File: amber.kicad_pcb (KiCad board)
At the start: 2 copper layers, 118.9 x 112.3 mm, 50 parts, among them J1 SJ-43504-SMT-TR

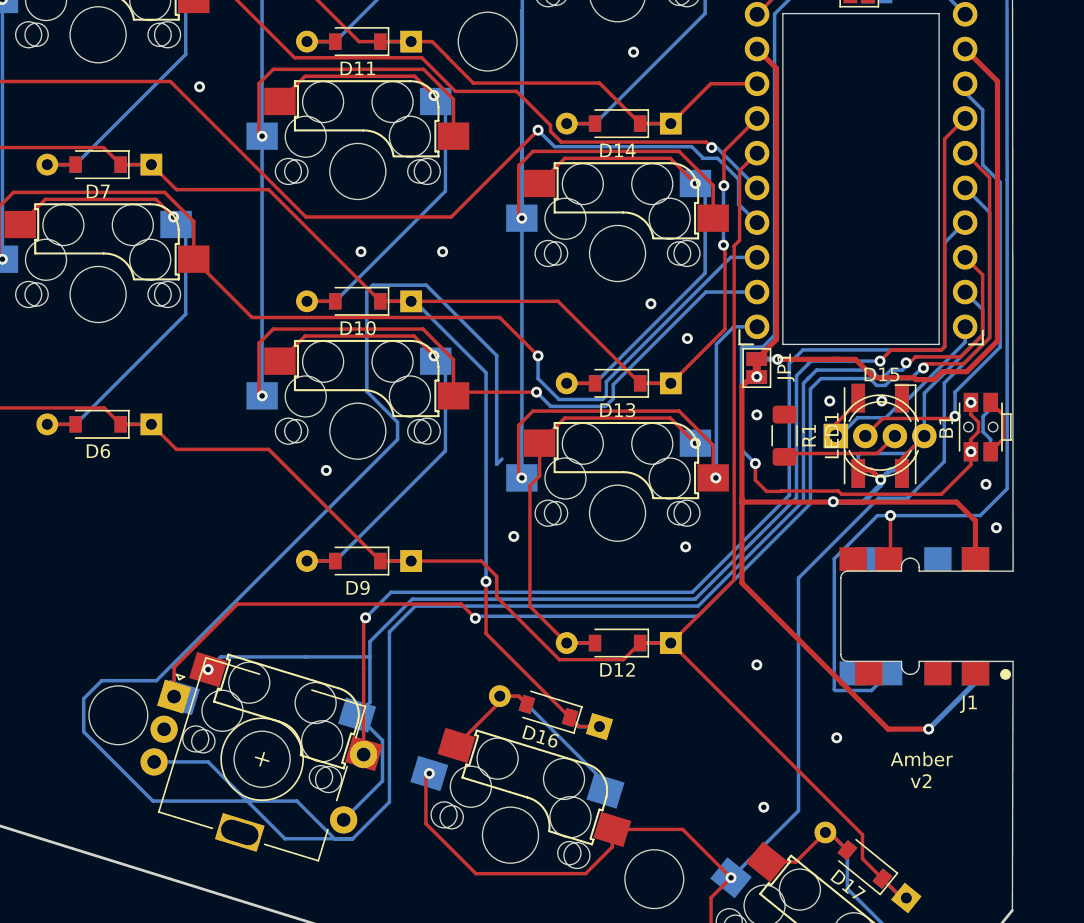
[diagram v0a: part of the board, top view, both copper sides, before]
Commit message: Cleanup tracks
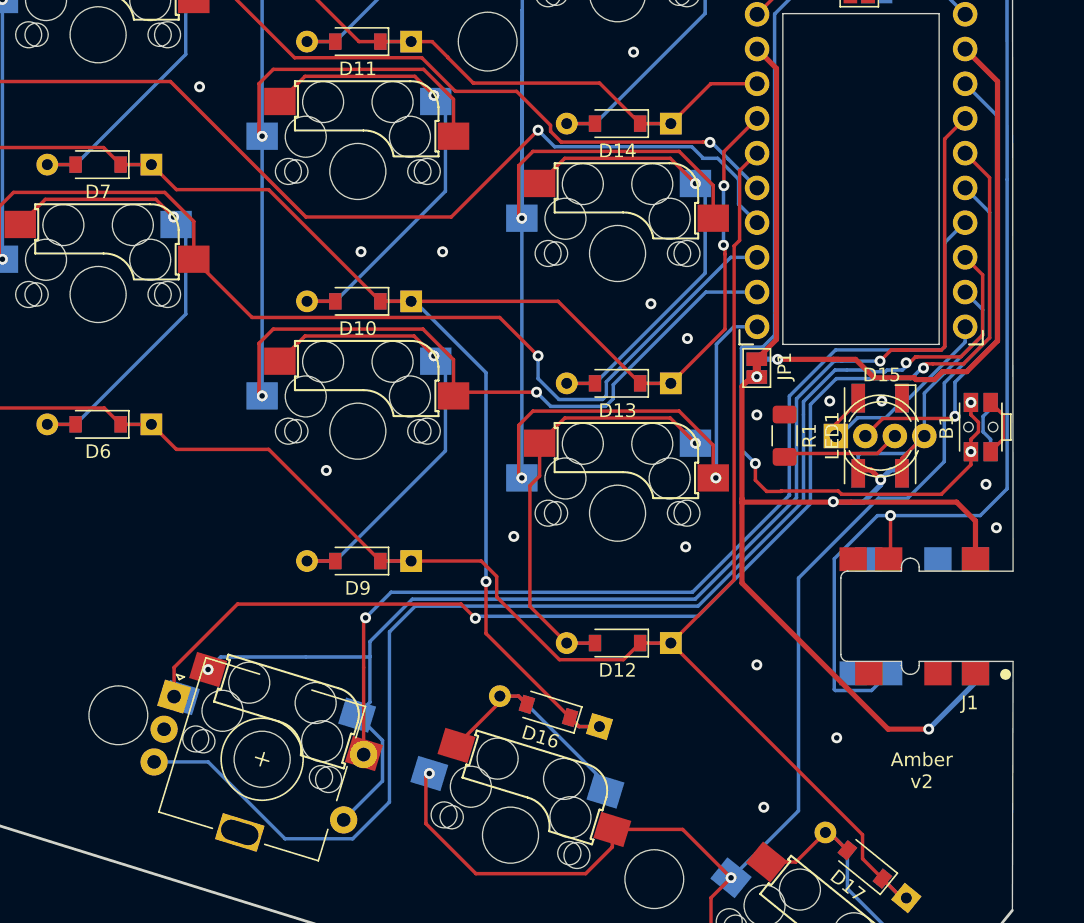
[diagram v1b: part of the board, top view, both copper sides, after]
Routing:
- net EB: track 185.7 -> 96.2 mm
- net RE: track 75.8 -> 74.4 mm
- net EA: track 92.2 -> 91.1 mm
- net CE: track 101.9 -> 100.9 mm
